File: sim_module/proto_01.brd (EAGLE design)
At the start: 64.4 x 44.4 mm, 4 parts, among them IC1 SIM900

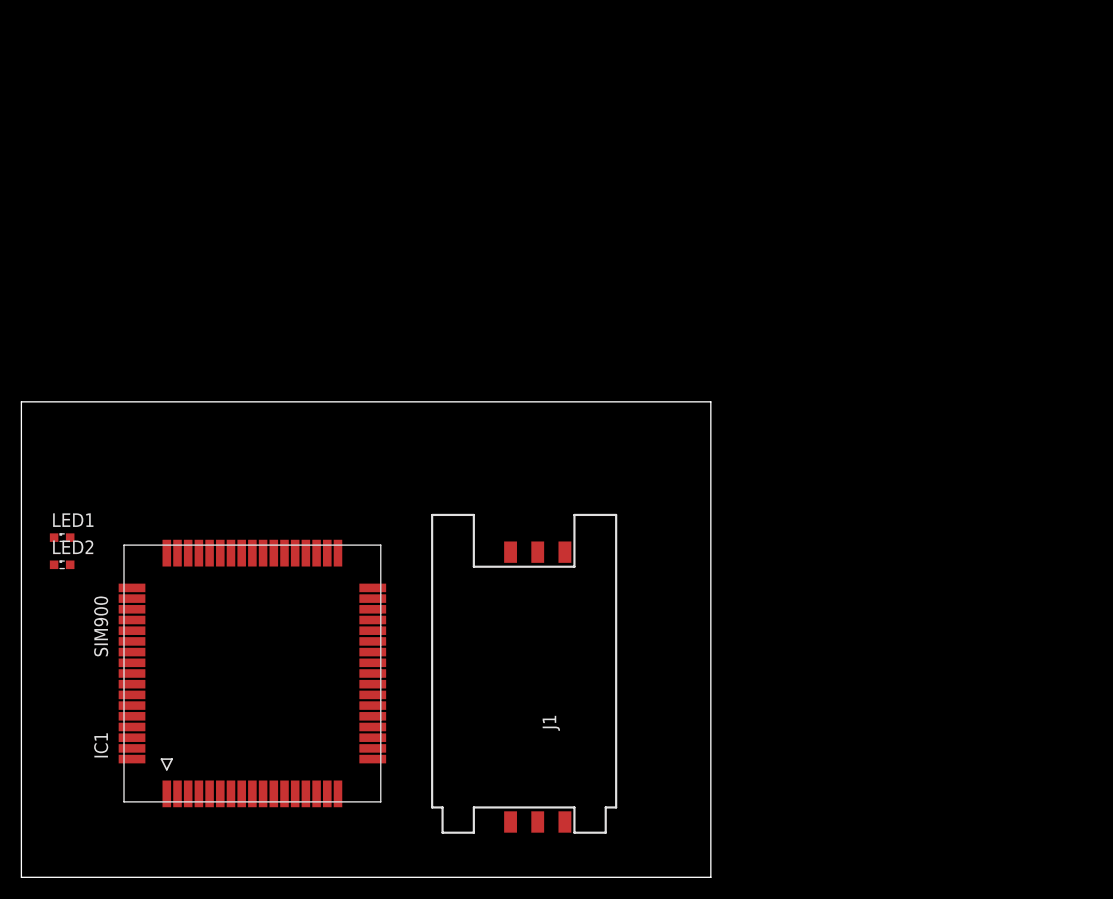
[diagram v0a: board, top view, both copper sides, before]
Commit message: Tried to do board for schematics
Tried to do board for schematics
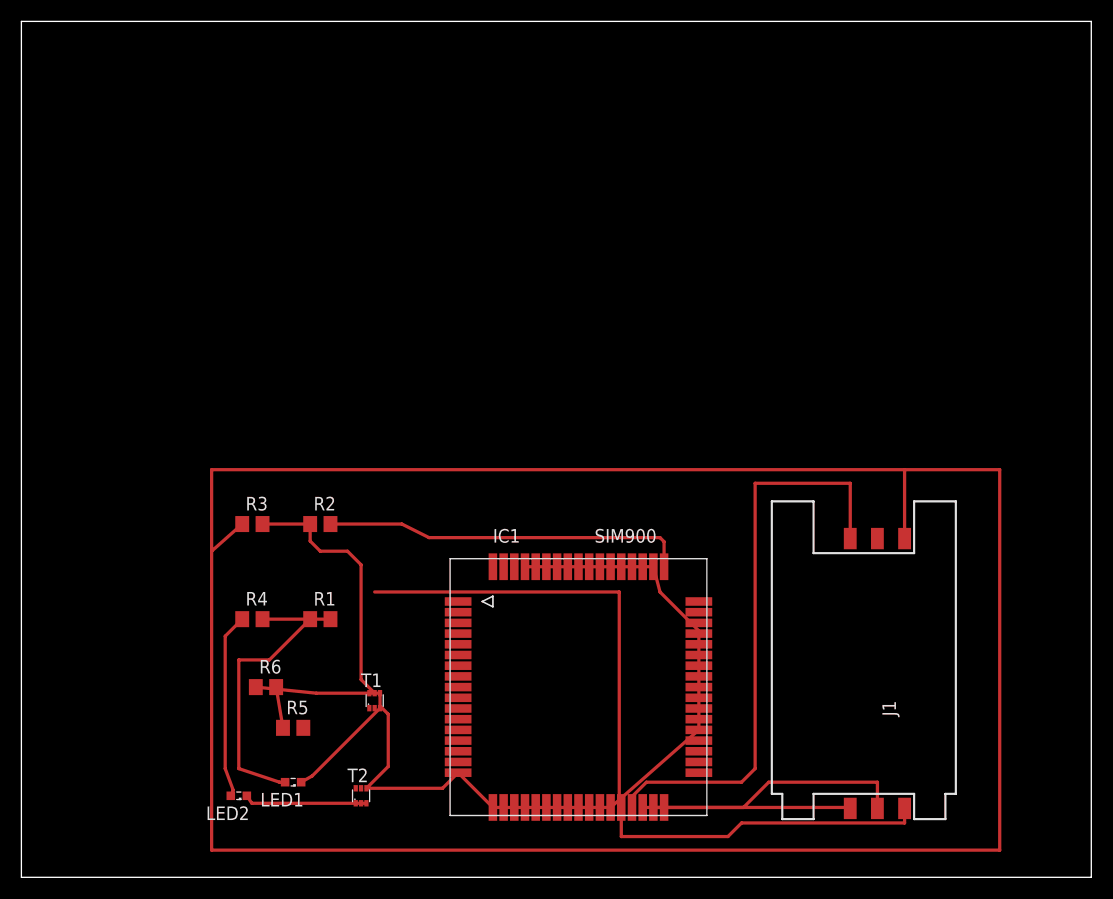
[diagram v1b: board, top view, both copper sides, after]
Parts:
- added R1, R4: 1k, resistor:R0805
- added R2, R5: 4.7k, resistor:R0805
- added R3, R6: 47k, resistor:R0805
- added T1, T2: CMLT5088E, transistor-neu-to92:SOT563
- moved J1 31.8 mm to (78.7, 19.1)
- moved LED1 31.4 mm to (25.4, 8.89), turned to 180 degrees
- moved IC1 30.5 mm to (52.1, 17.8), turned to 0 degrees
- moved LED2 27.2 mm to (20.3, 7.62), turned to 180 degrees
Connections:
- new net N$10: LED2.A, R4.1
- new net N$11: R5.1, R6.2, T2.5
- new net N$6: LED1.C, T1.3
- new net N$7: LED1.A, R1.1
- new net N$8: R2.1, R3.2, T1.5
- new net N$9: LED2.C, T2.3
- new net NETLIGHT: IC1.52, R2.2
- new net STATUS: IC1.66, R5.2
- net GND: now also R3.1, R6.1, T1.4, T2.4
- net SIM_VDD: now also R1.2, R4.2
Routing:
- net GND: track 0.00 -> 315.0 mm
- net SIM_VDD: track 0.00 -> 80.5 mm
- net SIM_DATA: track 0.00 -> 54.3 mm
- net NETLIGHT: track 0.00 -> 34.0 mm
- net SIM_RST: track 0.00 -> 24.4 mm
- net N$8: track 0.00 -> 24.2 mm
- net N$7: track 0.00 -> 22.9 mm
- net SIM_CLK: track 0.00 -> 19.4 mm
- net N$10: track 0.00 -> 17.4 mm
- net N$9: track 0.00 -> 11.6 mm
- net N$6: track 0.00 -> 10.1 mm
- net N$11: track 0.00 -> 3.86 mm
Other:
- board size 64.4 x 44.4 mm -> 100 x 80 mm
